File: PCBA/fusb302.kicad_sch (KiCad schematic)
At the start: 3 parts, among them U401 FUSB302B

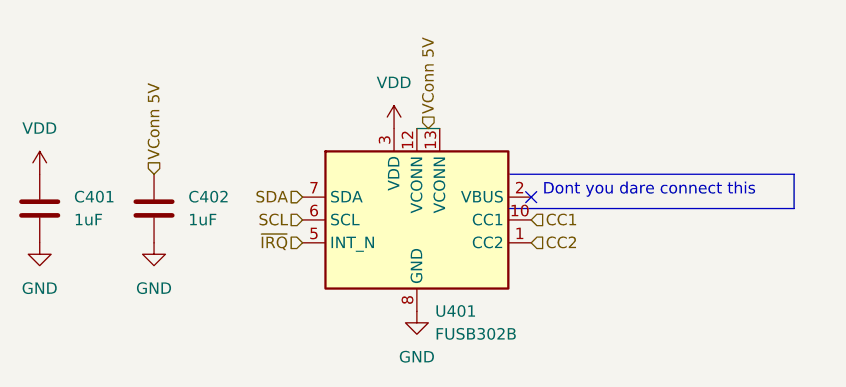
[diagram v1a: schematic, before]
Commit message: .
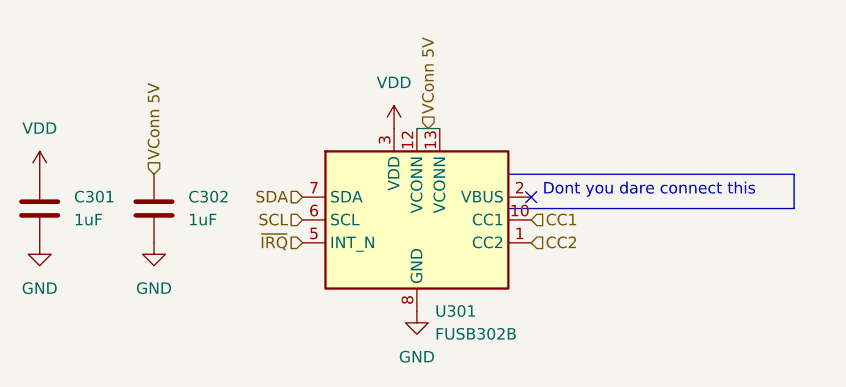
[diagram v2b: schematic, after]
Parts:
- renumbered C401 to C301, C402 to C302, U401 to U301
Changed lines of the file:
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@@
   (symbol (lib_id "Device:C") (at 88.9 85.09 0)
     (in_bom yes) (on_board yes) (fields_autoplaced)
-    (property "Reference" "C401" (id 0) (at 92.71 83.8199 0)
+    (property "Reference" "C301" (id 0) (at 92.71 83.8199 0)
       (effects (font (size 1.27 1.27)) (justify left))
     )
@@
   (symbol (lib_id "power:GND") (at 101.6 88.9 0)
     (in_bom yes) (on_board yes) (fields_autoplaced)
-    (property "Reference" "#PWR0124" (id 0) (at 101.6 95.25 0)
+    (property "Reference" "#PWR0110" (id 0) (at 101.6 95.25 0)
       (effects (font (size 1.27 1.27)) hide)
     )
@@
   (symbol (lib_id "power:VDD") (at 88.9 81.28 0)
     (in_bom yes) (on_board yes) (fields_autoplaced)
-    (property "Reference" "#PWR0126" (id 0) (at 88.9 85.09 0)
+    (property "Reference" "#PWR0111" (id 0) (at 88.9 85.09 0)
       (effects (font (size 1.27 1.27)) hide)
     )
@@
   (symbol (lib_id "power:GND") (at 88.9 88.9 0)
     (in_bom yes) (on_board yes) (fields_autoplaced)
-    (property "Reference" "#PWR0125" (id 0) (at 88.9 95.25 0)
+    (property "Reference" "#PWR0112" (id 0) (at 88.9 95.25 0)
       (effects (font (size 1.27 1.27)) hide)
     )
@@
   (symbol (lib_id "power:GND") (at 130.81 96.52 0)
     (in_bom yes) (on_board yes) (fields_autoplaced)
-    (property "Reference" "#PWR0122" (id 0) (at 130.81 102.87 0)
+    (property "Reference" "#PWR0109" (id 0) (at 130.81 102.87 0)
       (effects (font (size 1.27 1.27)) hide)
     )
@@
   (symbol (lib_id "Device:C") (at 101.6 85.09 0)
     (in_bom yes) (on_board yes) (fields_autoplaced)
-    (property "Reference" "C402" (id 0) (at 105.41 83.8199 0)
+    (property "Reference" "C302" (id 0) (at 105.41 83.8199 0)
       (effects (font (size 1.27 1.27)) (justify left))
     )
@@
   (symbol (lib_id "power:VDD") (at 128.27 76.2 0)
     (in_bom yes) (on_board yes) (fields_autoplaced)
-    (property "Reference" "#PWR0123" (id 0) (at 128.27 80.01 0)
+    (property "Reference" "#PWR0113" (id 0) (at 128.27 80.01 0)
       (effects (font (size 1.27 1.27)) hide)
     )
@@
   (symbol (lib_id "Interface_USB:FUSB302B01MPX") (at 130.81 86.36 0)
     (in_bom yes) (on_board yes) (fields_autoplaced)
-    (property "Reference" "U401" (id 0) (at 132.8294 96.52 0)
+    (property "Reference" "U301" (id 0) (at 132.8294 96.52 0)
       (effects (font (size 1.27 1.27)) (justify left))
     )

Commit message: Rough outline
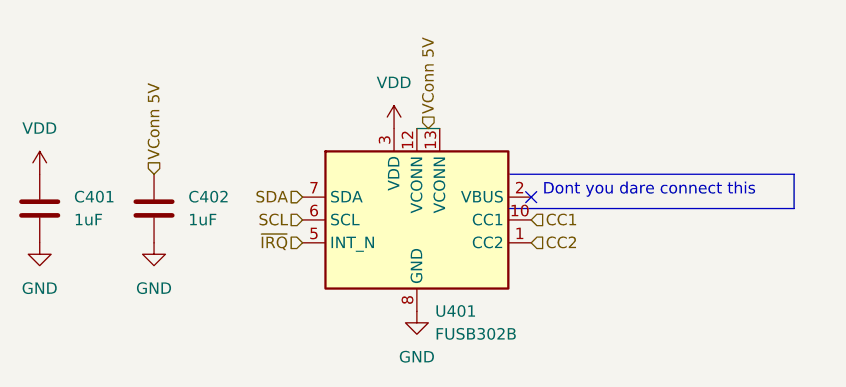
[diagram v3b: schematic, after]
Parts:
- renumbered C301 to C401, C302 to C402, U301 to U401
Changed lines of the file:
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@@
   (symbol (lib_id "Device:C") (at 88.9 85.09 0)
     (in_bom yes) (on_board yes) (fields_autoplaced)
-    (property "Reference" "C301" (id 0) (at 92.71 83.8199 0)
+    (property "Reference" "C401" (id 0) (at 92.71 83.8199 0)
       (effects (font (size 1.27 1.27)) (justify left))
     )
@@
   (symbol (lib_id "power:GND") (at 101.6 88.9 0)
     (in_bom yes) (on_board yes) (fields_autoplaced)
-    (property "Reference" "#PWR0110" (id 0) (at 101.6 95.25 0)
+    (property "Reference" "#PWR0124" (id 0) (at 101.6 95.25 0)
       (effects (font (size 1.27 1.27)) hide)
     )
@@
   (symbol (lib_id "power:VDD") (at 88.9 81.28 0)
     (in_bom yes) (on_board yes) (fields_autoplaced)
-    (property "Reference" "#PWR0111" (id 0) (at 88.9 85.09 0)
+    (property "Reference" "#PWR0126" (id 0) (at 88.9 85.09 0)
       (effects (font (size 1.27 1.27)) hide)
     )
@@
   (symbol (lib_id "power:GND") (at 88.9 88.9 0)
     (in_bom yes) (on_board yes) (fields_autoplaced)
-    (property "Reference" "#PWR0112" (id 0) (at 88.9 95.25 0)
+    (property "Reference" "#PWR0125" (id 0) (at 88.9 95.25 0)
       (effects (font (size 1.27 1.27)) hide)
     )
@@
   (symbol (lib_id "power:GND") (at 130.81 96.52 0)
     (in_bom yes) (on_board yes) (fields_autoplaced)
-    (property "Reference" "#PWR0109" (id 0) (at 130.81 102.87 0)
+    (property "Reference" "#PWR0122" (id 0) (at 130.81 102.87 0)
       (effects (font (size 1.27 1.27)) hide)
     )
@@
   (symbol (lib_id "Device:C") (at 101.6 85.09 0)
     (in_bom yes) (on_board yes) (fields_autoplaced)
-    (property "Reference" "C302" (id 0) (at 105.41 83.8199 0)
+    (property "Reference" "C402" (id 0) (at 105.41 83.8199 0)
       (effects (font (size 1.27 1.27)) (justify left))
     )
@@
   (symbol (lib_id "power:VDD") (at 128.27 76.2 0)
     (in_bom yes) (on_board yes) (fields_autoplaced)
-    (property "Reference" "#PWR0113" (id 0) (at 128.27 80.01 0)
+    (property "Reference" "#PWR0123" (id 0) (at 128.27 80.01 0)
       (effects (font (size 1.27 1.27)) hide)
     )
@@
   (symbol (lib_id "Interface_USB:FUSB302B01MPX") (at 130.81 86.36 0)
     (in_bom yes) (on_board yes) (fields_autoplaced)
-    (property "Reference" "U301" (id 0) (at 132.8294 96.52 0)
+    (property "Reference" "U401" (id 0) (at 132.8294 96.52 0)
       (effects (font (size 1.27 1.27)) (justify left))
     )

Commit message: More rough placement
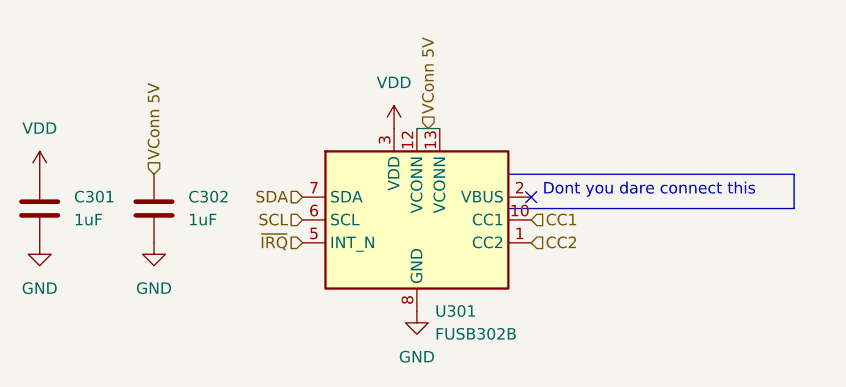
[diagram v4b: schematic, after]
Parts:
- renumbered C401 to C301, C402 to C302, U401 to U301
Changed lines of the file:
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@@
   (symbol (lib_id "Device:C") (at 88.9 85.09 0)
     (in_bom yes) (on_board yes) (fields_autoplaced)
-    (property "Reference" "C401" (id 0) (at 92.71 83.8199 0)
+    (property "Reference" "C301" (id 0) (at 92.71 83.8199 0)
       (effects (font (size 1.27 1.27)) (justify left))
     )
@@
   (symbol (lib_id "Device:C") (at 101.6 85.09 0)
     (in_bom yes) (on_board yes) (fields_autoplaced)
-    (property "Reference" "C402" (id 0) (at 105.41 83.8199 0)
+    (property "Reference" "C302" (id 0) (at 105.41 83.8199 0)
       (effects (font (size 1.27 1.27)) (justify left))
     )
@@
   (symbol (lib_id "Interface_USB:FUSB302B01MPX") (at 130.81 86.36 0)
     (in_bom yes) (on_board yes) (fields_autoplaced)
-    (property "Reference" "U401" (id 0) (at 132.8294 96.52 0)
+    (property "Reference" "U301" (id 0) (at 132.8294 96.52 0)
       (effects (font (size 1.27 1.27)) (justify left))
     )

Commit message: Routing
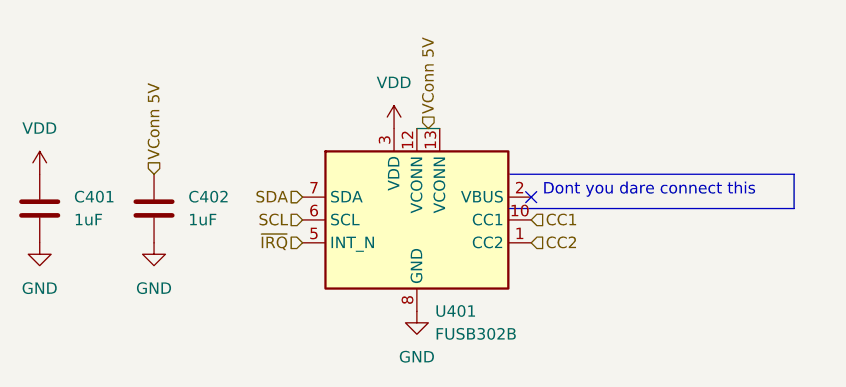
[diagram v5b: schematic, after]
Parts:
- renumbered C301 to C401, C302 to C402, U301 to U401
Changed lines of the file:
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@@
   (symbol (lib_id "Device:C") (at 88.9 85.09 0)
     (in_bom yes) (on_board yes) (fields_autoplaced)
-    (property "Reference" "C301" (id 0) (at 92.71 83.8199 0)
+    (property "Reference" "C401" (id 0) (at 92.71 83.8199 0)
       (effects (font (size 1.27 1.27)) (justify left))
     )
@@
   (symbol (lib_id "Device:C") (at 101.6 85.09 0)
     (in_bom yes) (on_board yes) (fields_autoplaced)
-    (property "Reference" "C302" (id 0) (at 105.41 83.8199 0)
+    (property "Reference" "C402" (id 0) (at 105.41 83.8199 0)
       (effects (font (size 1.27 1.27)) (justify left))
     )
@@
   (symbol (lib_id "Interface_USB:FUSB302B01MPX") (at 130.81 86.36 0)
     (in_bom yes) (on_board yes) (fields_autoplaced)
-    (property "Reference" "U301" (id 0) (at 132.8294 96.52 0)
+    (property "Reference" "U401" (id 0) (at 132.8294 96.52 0)
       (effects (font (size 1.27 1.27)) (justify left))
     )
